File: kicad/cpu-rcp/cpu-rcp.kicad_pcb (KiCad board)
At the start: 4 copper layers, 90.2 x 57.1 mm, 77 parts, among them P1 RDRAM-EDGE, P5 502790-5091, SW1 Reset, U10 CPU-NUS, U3 U3, U6 PIF-NUS, U7 MX8330, U8 LC125, U9 RCP-NUS, X1 14.318MHz

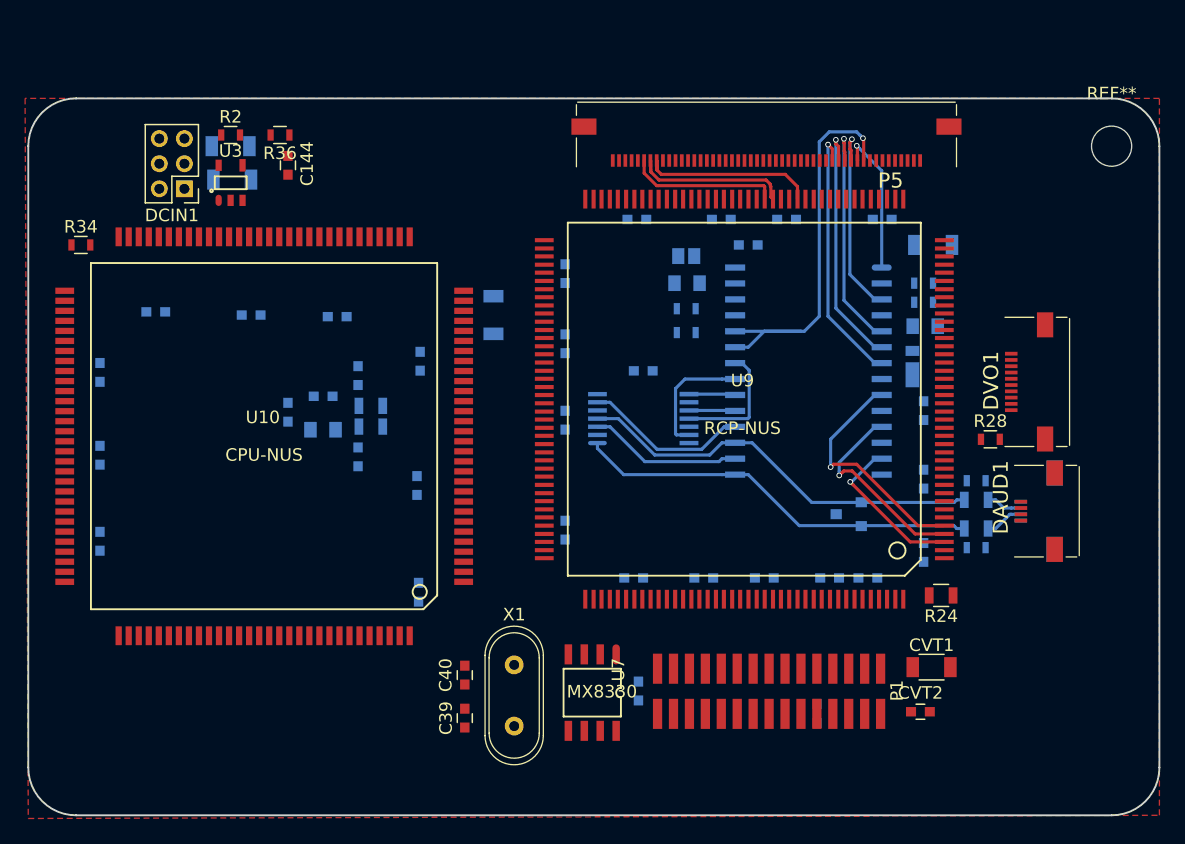
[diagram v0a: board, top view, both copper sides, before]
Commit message: WIP
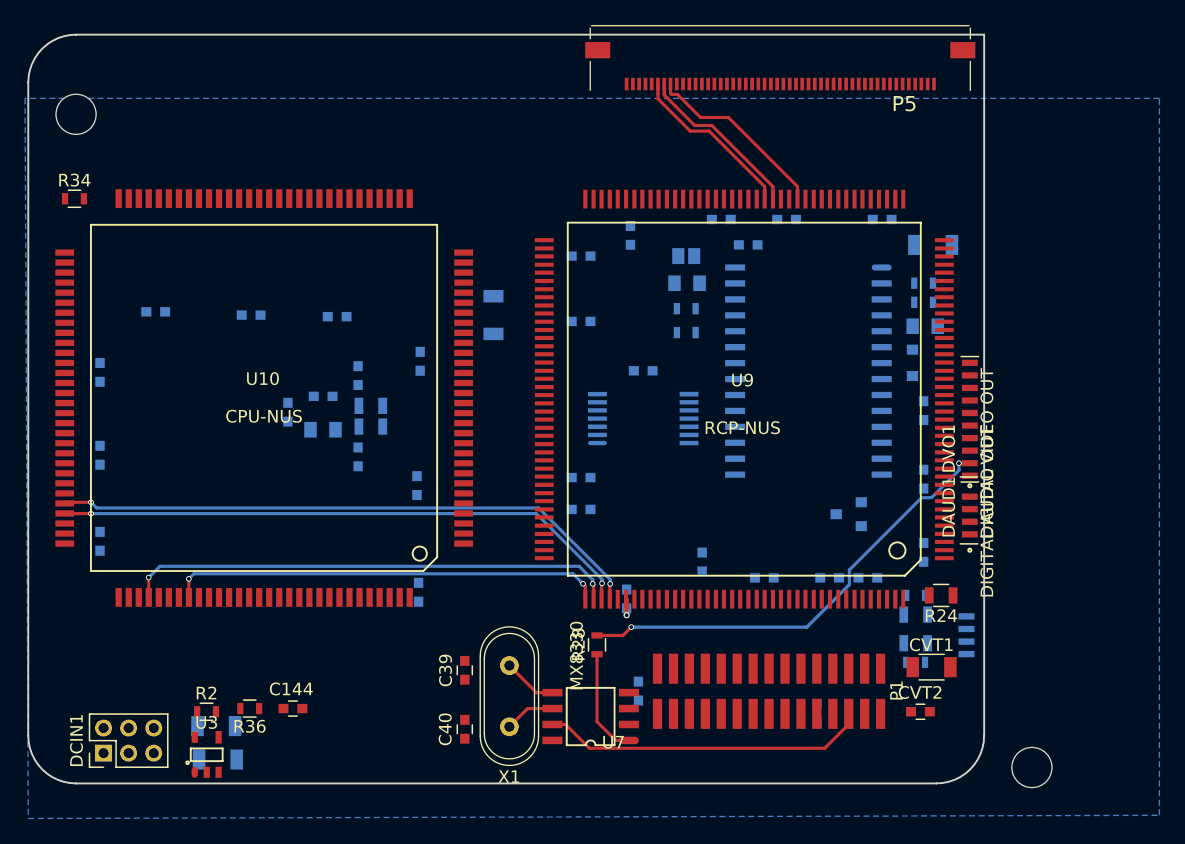
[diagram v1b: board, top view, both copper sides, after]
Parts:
- added REF**: MountingHole_3.2mm_M3, Mounting_Holes:MountingHole_3.2mm_M3, F.Cu at (105.4, 78.7)
- D2: footprint n64:D_TUMD2 -> n64:D_0805
- DAUD1, JOY1: footprint n64:connector-molex-505110-0492 -> n64:Connectors_GS4
- DVO1: footprint n64:connector-molex-505110-1092 -> n64:Connectors_GS10
- moved REF** 82.6 mm to (29.2, 26.7)
- moved C73 46.2 mm to (40.5, 78.1)
- moved C142 46.2 mm to (40.4, 75.4)
- moved R2 46.0 mm to (39.6, 74.3)
- moved R36 45.8 mm to (43.1, 74.0)
- moved U3 45.6 mm to (39.6, 77.7)
- moved DCIN1 45.4 mm to (31.4, 77.6), turned to 90 degrees
- moved C144 43.3 mm to (46.5, 74.0), turned to 0 degrees
- moved R28 35.4 mm to (70.7, 69.0), turned to 90 degrees
- moved FIL2 10.3 mm to (96.1, 68.8)
- moved R37 10.3 mm to (96.1, 70.4)
- moved FIL4 10.3 mm to (96.1, 66.5)
- moved JOY1 10.3 mm to (100.2, 66.7)
- moved R38 10.3 mm to (96.1, 65.0)
- moved DVO1 6.47 mm to (100.5, 55.5)
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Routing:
- net /SYSAD28: track 0.00 -> 47.6 mm, vias 0 -> 2
- net /SYSAD27: track 0.00 -> 46.6 mm, vias 0 -> 2
- net /SYSAD26: track 0.00 -> 39.4 mm, vias 0 -> 2
- net Net-(DVO1-Pad2): track 0.00 -> 36.4 mm, vias 0 -> 2
- net /SYSAD25: track 0.00 -> 34.7 mm, vias 0 -> 2
- net JOY2_DATA: track 32.9 -> 0.00 mm
- net JOY1_DATA: track 32.9 -> 0.00 mm
- net EEPROM_DAT: track 32.7 -> 0.00 mm, vias 1 -> 0
- net ENABLE_CLK: track 0.00 -> 26.0 mm
- net /NMI: track 20.9 -> 0.00 mm, vias 1 -> 0
- net /COLDRESET: track 20.2 -> 0.00 mm, vias 1 -> 0
- net PIF_CLK: track 18.9 -> 0.00 mm, vias 1 -> 0
- net CIC_IN: track 18.7 -> 0.00 mm, vias 1 -> 0
- net PIF_ADR: track 16.2 -> 0.00 mm, vias 1 -> 0
- net CIC_OUT: track 16.0 -> 0.00 mm, vias 1 -> 0
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- added copper zone on B.Cu, net GND
- removed copper zone on F.Cu, net GND
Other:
- board size 90.2 x 57.1 mm -> 76.2 x 59.7 mm
